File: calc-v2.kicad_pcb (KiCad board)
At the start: 2 copper layers, 32 parts, among them U1 W25Q128JVS, U2 NCP1117-3.3_SOT223, U3 BQ24074RGT, U4 TPS61165DBV, U5 RP2350B, U6 APS6404L-3SQRx-ZR

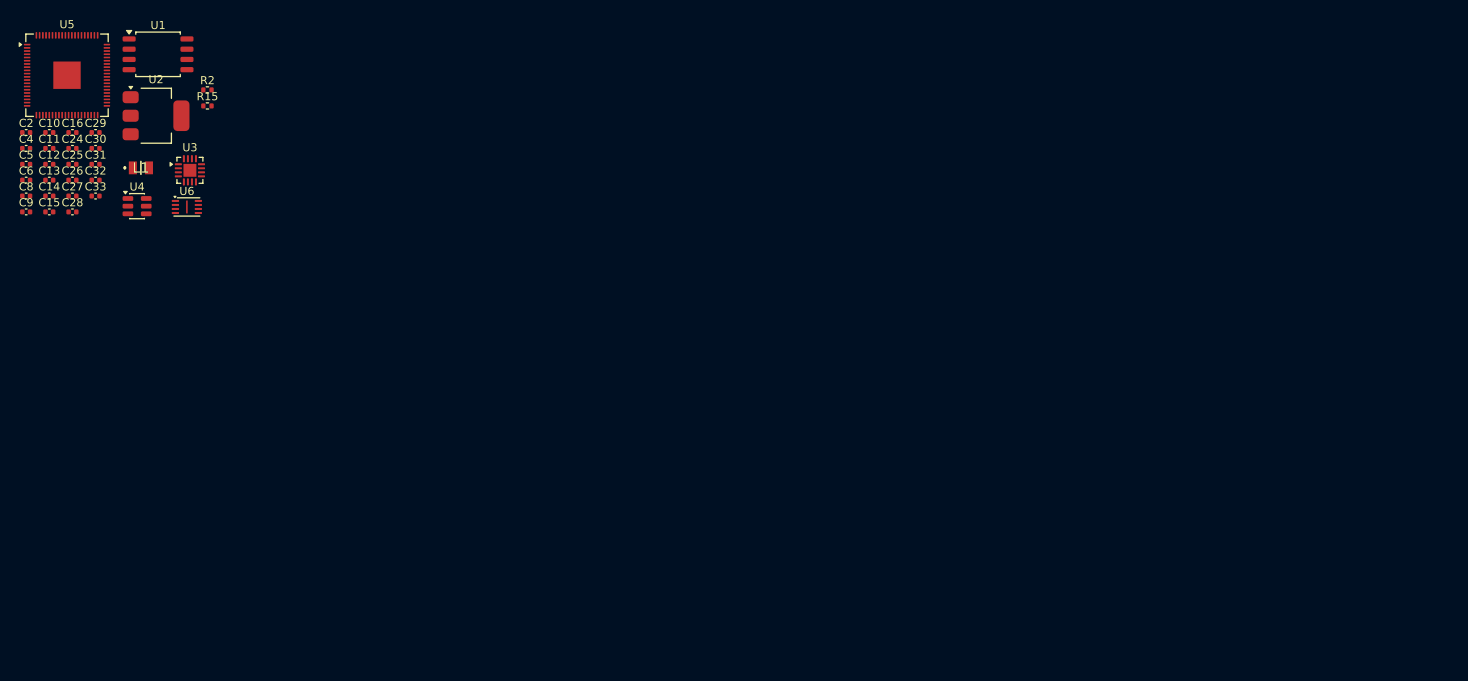
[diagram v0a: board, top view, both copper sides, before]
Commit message: more changes
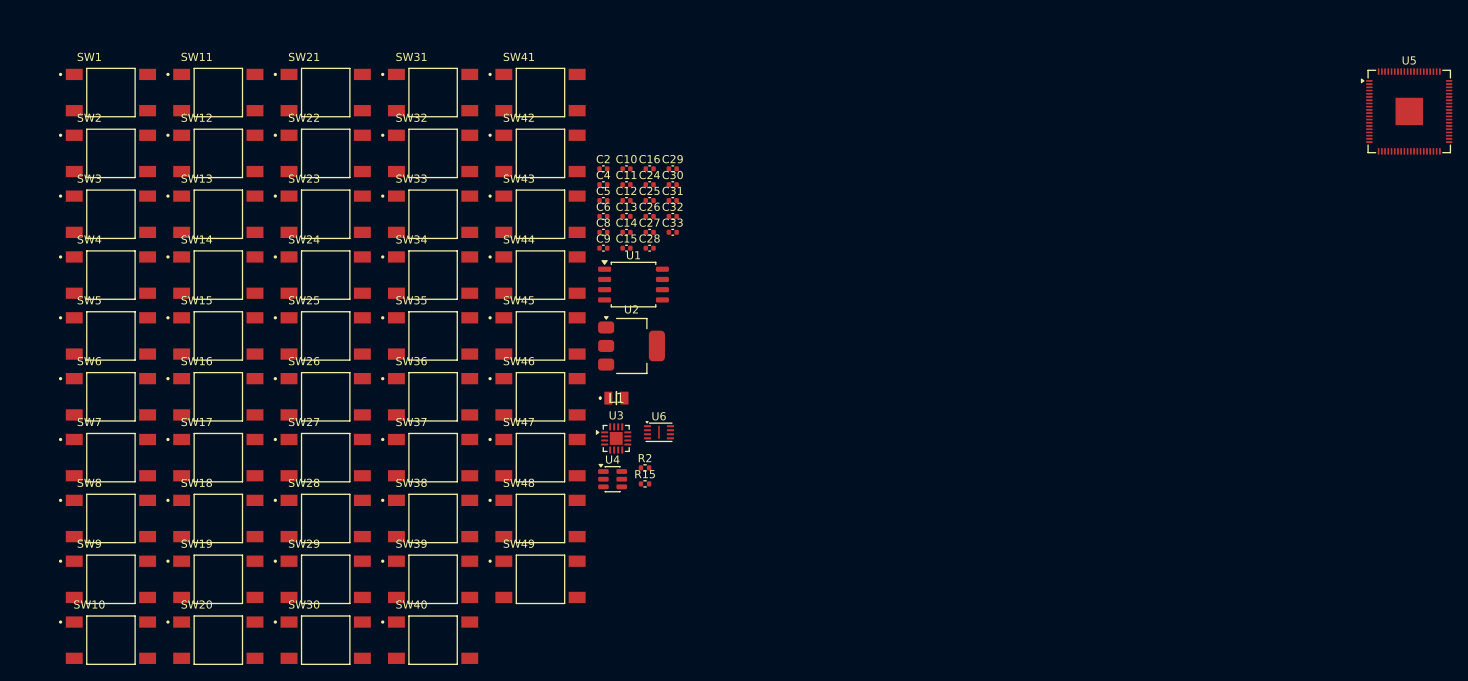
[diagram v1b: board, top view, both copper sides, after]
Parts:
- added SW1: TS04-66-43-BK-100-SMT, AAAAA:SW_TS04-66-43-BK-100-SMT, F.Cu at (23.9, 20.3)
- added SW10: TS04-66-43-BK-100-SMT, AAAAA:SW_TS04-66-43-BK-100-SMT, F.Cu at (23.9, 88.2)
- added SW11: TS04-66-43-BK-100-SMT, AAAAA:SW_TS04-66-43-BK-100-SMT, F.Cu at (37.3, 20.3)
- added SW12: TS04-66-43-BK-100-SMT, AAAAA:SW_TS04-66-43-BK-100-SMT, F.Cu at (37.3, 27.8)
- added SW13: TS04-66-43-BK-100-SMT, AAAAA:SW_TS04-66-43-BK-100-SMT, F.Cu at (37.3, 35.4)
- added SW14: TS04-66-43-BK-100-SMT, AAAAA:SW_TS04-66-43-BK-100-SMT, F.Cu at (37.3, 42.9)
- added SW15: TS04-66-43-BK-100-SMT, AAAAA:SW_TS04-66-43-BK-100-SMT, F.Cu at (37.3, 50.5)
- added SW16: TS04-66-43-BK-100-SMT, AAAAA:SW_TS04-66-43-BK-100-SMT, F.Cu at (37.3, 58.0)
- added SW17: TS04-66-43-BK-100-SMT, AAAAA:SW_TS04-66-43-BK-100-SMT, F.Cu at (37.3, 65.6)
- added SW18: TS04-66-43-BK-100-SMT, AAAAA:SW_TS04-66-43-BK-100-SMT, F.Cu at (37.3, 73.1)
- added SW19: TS04-66-43-BK-100-SMT, AAAAA:SW_TS04-66-43-BK-100-SMT, F.Cu at (37.3, 80.7)
- added SW2: TS04-66-43-BK-100-SMT, AAAAA:SW_TS04-66-43-BK-100-SMT, F.Cu at (23.9, 27.8)
- added SW20: TS04-66-43-BK-100-SMT, AAAAA:SW_TS04-66-43-BK-100-SMT, F.Cu at (37.3, 88.2)
- added SW21: TS04-66-43-BK-100-SMT, AAAAA:SW_TS04-66-43-BK-100-SMT, F.Cu at (50.6, 20.3)
- added SW22: TS04-66-43-BK-100-SMT, AAAAA:SW_TS04-66-43-BK-100-SMT, F.Cu at (50.6, 27.8)
- added SW23: TS04-66-43-BK-100-SMT, AAAAA:SW_TS04-66-43-BK-100-SMT, F.Cu at (50.6, 35.4)
- added SW24: TS04-66-43-BK-100-SMT, AAAAA:SW_TS04-66-43-BK-100-SMT, F.Cu at (50.6, 42.9)
- added SW25: TS04-66-43-BK-100-SMT, AAAAA:SW_TS04-66-43-BK-100-SMT, F.Cu at (50.6, 50.5)
- added SW26: TS04-66-43-BK-100-SMT, AAAAA:SW_TS04-66-43-BK-100-SMT, F.Cu at (50.6, 58.0)
- added SW27: TS04-66-43-BK-100-SMT, AAAAA:SW_TS04-66-43-BK-100-SMT, F.Cu at (50.6, 65.6)
- added SW28: TS04-66-43-BK-100-SMT, AAAAA:SW_TS04-66-43-BK-100-SMT, F.Cu at (50.6, 73.1)
- added SW29: TS04-66-43-BK-100-SMT, AAAAA:SW_TS04-66-43-BK-100-SMT, F.Cu at (50.6, 80.7)
- added SW3: TS04-66-43-BK-100-SMT, AAAAA:SW_TS04-66-43-BK-100-SMT, F.Cu at (23.9, 35.4)
- added SW30: TS04-66-43-BK-100-SMT, AAAAA:SW_TS04-66-43-BK-100-SMT, F.Cu at (50.6, 88.2)
- added SW31: TS04-66-43-BK-100-SMT, AAAAA:SW_TS04-66-43-BK-100-SMT, F.Cu at (63.9, 20.3)
- added SW32: TS04-66-43-BK-100-SMT, AAAAA:SW_TS04-66-43-BK-100-SMT, F.Cu at (63.9, 27.8)
- added SW33: TS04-66-43-BK-100-SMT, AAAAA:SW_TS04-66-43-BK-100-SMT, F.Cu at (63.9, 35.4)
- added SW34: TS04-66-43-BK-100-SMT, AAAAA:SW_TS04-66-43-BK-100-SMT, F.Cu at (63.9, 42.9)
- added SW35: TS04-66-43-BK-100-SMT, AAAAA:SW_TS04-66-43-BK-100-SMT, F.Cu at (63.9, 50.5)
- added SW36: TS04-66-43-BK-100-SMT, AAAAA:SW_TS04-66-43-BK-100-SMT, F.Cu at (63.9, 58.0)
- added SW37: TS04-66-43-BK-100-SMT, AAAAA:SW_TS04-66-43-BK-100-SMT, F.Cu at (63.9, 65.6)
- added SW38: TS04-66-43-BK-100-SMT, AAAAA:SW_TS04-66-43-BK-100-SMT, F.Cu at (63.9, 73.1)
- added SW39: TS04-66-43-BK-100-SMT, AAAAA:SW_TS04-66-43-BK-100-SMT, F.Cu at (63.9, 80.7)
- added SW4: TS04-66-43-BK-100-SMT, AAAAA:SW_TS04-66-43-BK-100-SMT, F.Cu at (23.9, 42.9)
- added SW40: TS04-66-43-BK-100-SMT, AAAAA:SW_TS04-66-43-BK-100-SMT, F.Cu at (63.9, 88.2)
- added SW41: TS04-66-43-BK-100-SMT, AAAAA:SW_TS04-66-43-BK-100-SMT, F.Cu at (77.2, 20.3)
- added SW42: TS04-66-43-BK-100-SMT, AAAAA:SW_TS04-66-43-BK-100-SMT, F.Cu at (77.2, 27.8)
- added SW43: TS04-66-43-BK-100-SMT, AAAAA:SW_TS04-66-43-BK-100-SMT, F.Cu at (77.2, 35.4)
- added SW44: TS04-66-43-BK-100-SMT, AAAAA:SW_TS04-66-43-BK-100-SMT, F.Cu at (77.2, 42.9)
- added SW45: TS04-66-43-BK-100-SMT, AAAAA:SW_TS04-66-43-BK-100-SMT, F.Cu at (77.2, 50.5)
- added SW46: TS04-66-43-BK-100-SMT, AAAAA:SW_TS04-66-43-BK-100-SMT, F.Cu at (77.2, 58.0)
- added SW47: TS04-66-43-BK-100-SMT, AAAAA:SW_TS04-66-43-BK-100-SMT, F.Cu at (77.2, 65.6)
- added SW48: TS04-66-43-BK-100-SMT, AAAAA:SW_TS04-66-43-BK-100-SMT, F.Cu at (77.2, 73.1)
- added SW49: SW_Push_45deg, AAAAA:SW_TS04-66-43-BK-100-SMT, F.Cu at (77.2, 80.7)
- added SW5: TS04-66-43-BK-100-SMT, AAAAA:SW_TS04-66-43-BK-100-SMT, F.Cu at (23.9, 50.5)
- added SW6: TS04-66-43-BK-100-SMT, AAAAA:SW_TS04-66-43-BK-100-SMT, F.Cu at (23.9, 58.0)
- added SW7: TS04-66-43-BK-100-SMT, AAAAA:SW_TS04-66-43-BK-100-SMT, F.Cu at (23.9, 65.6)
- added SW8: TS04-66-43-BK-100-SMT, AAAAA:SW_TS04-66-43-BK-100-SMT, F.Cu at (23.9, 73.1)
- added SW9: TS04-66-43-BK-100-SMT, AAAAA:SW_TS04-66-43-BK-100-SMT, F.Cu at (23.9, 80.7)
- moved U5 166.6 mm to (185.1, 22.6)
- moved C10 71.8 mm to (87.9, 29.7)
- moved C11 71.8 mm to (87.9, 31.7)
- moved C12 71.8 mm to (87.9, 33.7)
- moved C13 71.8 mm to (87.9, 35.6)
- moved C14 71.8 mm to (87.9, 37.6)
- moved C15 71.8 mm to (87.9, 39.6)
- moved C16 71.8 mm to (90.8, 29.7)
- moved C2 71.8 mm to (85.1, 29.7)
- moved C24 71.8 mm to (90.8, 31.7)
- moved C25 71.8 mm to (90.8, 33.7)
- moved C26 71.8 mm to (90.8, 35.6)
- moved C27 71.8 mm to (90.8, 37.6)
- moved C28 71.8 mm to (90.8, 39.6)
- moved C29 71.8 mm to (93.7, 29.7)
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
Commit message: components
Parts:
- added C34: 1u, Capacitor_SMD:C_0402_1005Metric, F.Cu at (202.6, 60.5)
- SW1, SW10, SW11, SW12, SW13, SW14, SW15, SW16, SW17, SW18, SW19, SW2, SW20, SW21, SW22, SW23, SW24, SW25, SW26, SW27, SW28, SW29, SW3, SW30, SW31, SW32, SW33, SW34, SW35, SW36, SW37, SW38, SW39, SW4, SW40, SW41, SW42, SW43, SW44, SW45, SW46, SW47, SW48, SW5, SW6, SW7, SW8, SW9: value TS04-66-43-BK-100-SMT -> SW_Push_45deg
- moved SW43 233.3 mm to (310.4, 30.0)
- moved SW44 219.5 mm to (296.4, 30.0)
- moved SW45 206.0 mm to (282.3, 30.0)
- moved SW46 193.0 mm to (268.2, 30.0)
- moved SW47 180.4 mm to (254.1, 30.0)
- moved SW48 168.4 mm to (240.0, 30.0)
- moved SW36 125.1 mm to (181.4, 101.0)
- moved SW16 125.1 mm to (154.8, 101.0)
- moved SW26 125.1 mm to (168.1, 101.0)
- moved SW1 125.1 mm to (141.4, 63.3)
- moved SW10 125.1 mm to (141.4, 131.2)
- moved SW2 125.1 mm to (141.4, 70.8)
- moved SW3 125.1 mm to (141.4, 78.4)
- moved SW31 125.1 mm to (181.4, 63.3)
- moved SW32 125.1 mm to (181.4, 70.8)
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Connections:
- SW1 pad 2: Net-(SW1-Pad2) -> SW_R1
- SW10 pad 1: Net-(SW10-Pad1) -> SW_C4
- SW10 pad 2: Net-(SW10-Pad2) -> SW_R2
- SW11 pad 1: Net-(SW11-Pad1) -> SW_C5
- SW11 pad 2: Net-(SW11-Pad2) -> SW_R2
- SW12 pad 2: unconnected-(SW12-Pad2) -> SW_R2
- SW13 pad 1: Net-(SW13-Pad1) -> SW_C1
- SW13 pad 2: Net-(SW13-Pad2) -> SW_R3
- SW14 pad 1: Net-(SW14-Pad1) -> SW_C2
- SW14 pad 2: Net-(SW14-Pad2) -> SW_R3
- SW15 pad 1: Net-(SW15-Pad1) -> SW_C3
- SW15 pad 2: Net-(SW15-Pad2) -> SW_R3
- SW16 pad 1: Net-(SW10-Pad3) -> SW_C4
- SW16 pad 2: Net-(SW16-Pad2) -> SW_R3
- SW17 pad 1: Net-(SW11-Pad3) -> SW_C5
- SW17 pad 2: Net-(SW17-Pad2) -> SW_R3
- SW18 pad 1: Net-(SW12-Pad3) -> Net-(SW12-Pad1)
- SW18 pad 2: unconnected-(SW18-Pad2) -> SW_R3
- SW19 pad 1: Net-(SW13-Pad3) -> SW_C1
- SW19 pad 2: Net-(SW19-Pad2) -> SW_R4
- SW2 pad 2: Net-(SW2-Pad2) -> SW_R1
- SW20 pad 1: Net-(SW14-Pad3) -> SW_C2
- SW20 pad 2: Net-(SW20-Pad2) -> SW_R4
- SW21 pad 1: Net-(SW15-Pad3) -> SW_C3
- SW21 pad 2: Net-(SW21-Pad2) -> SW_R4
- SW22 pad 1: Net-(SW16-Pad3) -> SW_C4
- SW22 pad 2: Net-(SW22-Pad2) -> SW_R4
- SW23 pad 1: Net-(SW17-Pad3) -> SW_C5
- SW23 pad 2: Net-(SW23-Pad2) -> SW_R4
- SW24 pad 1: Net-(SW18-Pad3) -> Net-(SW12-Pad1)
- SW24 pad 2: unconnected-(SW24-Pad2) -> SW_R4
- SW25 pad 1: Net-(SW19-Pad3) -> SW_C1
- SW25 pad 2: Net-(SW25-Pad2) -> SW_R5
- SW26 pad 1: Net-(SW20-Pad3) -> SW_C2
- SW26 pad 2: Net-(SW26-Pad2) -> SW_R5
- SW27 pad 1: Net-(SW21-Pad3) -> SW_C3
- SW27 pad 2: Net-(SW27-Pad2) -> SW_R5
- SW28 pad 1: Net-(SW22-Pad3) -> SW_C4
- SW28 pad 2: Net-(SW28-Pad2) -> SW_R5
- SW29 pad 1: Net-(SW23-Pad3) -> SW_C5
- SW29 pad 2: Net-(SW29-Pad2) -> SW_R5
- SW3 pad 2: Net-(SW3-Pad2) -> SW_R1
- SW30 pad 1: Net-(SW24-Pad3) -> Net-(SW12-Pad1)
- SW30 pad 2: unconnected-(SW30-Pad2) -> SW_R5
- SW31 pad 1: Net-(SW25-Pad3) -> SW_C1
- SW31 pad 2: Net-(SW31-Pad2) -> SW_R6
- SW32 pad 1: Net-(SW26-Pad3) -> SW_C2
- SW32 pad 2: Net-(SW32-Pad2) -> SW_R6
- SW33 pad 1: Net-(SW27-Pad3) -> SW_C3
- SW33 pad 2: Net-(SW33-Pad2) -> SW_R6
- SW34 pad 1: Net-(SW28-Pad3) -> SW_C4
- SW34 pad 2: Net-(SW34-Pad2) -> SW_R6
- SW35 pad 1: Net-(SW29-Pad3) -> SW_C5
- SW35 pad 2: Net-(SW35-Pad2) -> SW_R6
- SW36 pad 1: Net-(SW30-Pad3) -> Net-(SW12-Pad1)
- SW36 pad 2: unconnected-(SW36-Pad2) -> SW_R6
- SW37 pad 1: Net-(SW31-Pad3) -> SW_C1
- SW37 pad 2: Net-(SW37-Pad2) -> SW_R7
- SW38 pad 1: Net-(SW32-Pad3) -> SW_C2
- SW38 pad 2: Net-(SW38-Pad2) -> SW_R7
- SW39 pad 1: Net-(SW33-Pad3) -> SW_C3
- SW39 pad 2: Net-(SW39-Pad2) -> SW_R7
- SW4 pad 2: Net-(SW4-Pad2) -> SW_R1
- SW40 pad 1: Net-(SW34-Pad3) -> SW_C4
- SW40 pad 2: Net-(SW40-Pad2) -> SW_R7
- SW41 pad 1: Net-(SW35-Pad3) -> SW_C5
- SW41 pad 2: Net-(SW41-Pad2) -> SW_R7
- SW42 pad 1: Net-(SW36-Pad3) -> Net-(SW12-Pad1)
- SW42 pad 2: unconnected-(SW42-Pad2) -> SW_R7
- SW43 pad 1: Net-(SW37-Pad3) -> SW_C1
- SW43 pad 2: Net-(SW43-Pad2) -> SW_R8
- SW44 pad 1: Net-(SW38-Pad3) -> SW_C2
- SW44 pad 2: Net-(SW44-Pad2) -> SW_R8
- SW45 pad 1: Net-(SW39-Pad3) -> SW_C3
- SW45 pad 2: Net-(SW45-Pad2) -> SW_R8
- SW46 pad 1: Net-(SW40-Pad3) -> SW_C4
- SW46 pad 2: Net-(SW46-Pad2) -> SW_R8
- SW47 pad 1: Net-(SW41-Pad3) -> SW_C5
- SW47 pad 2: Net-(SW47-Pad2) -> SW_R8
- SW48 pad 1: Net-(SW42-Pad3) -> Net-(SW12-Pad1)
- SW48 pad 2: unconnected-(SW48-Pad2) -> SW_R8
- SW5 pad 2: Net-(SW5-Pad2) -> SW_R1
- SW6 pad 1: SW_C6 -> Net-(SW12-Pad1)
- SW6 pad 2: unconnected-(SW6-Pad2) -> SW_R1
- SW7 pad 1: Net-(SW1-Pad3) -> SW_C1
- SW7 pad 2: Net-(SW7-Pad2) -> SW_R2
- SW8 pad 1: Net-(SW2-Pad3) -> SW_C2
- SW8 pad 2: Net-(SW8-Pad2) -> SW_R2
- SW9 pad 1: Net-(SW3-Pad3) -> SW_C3
- SW9 pad 2: Net-(SW10-Pad4) -> SW_R2
- U3 pad 13: unconnected-(U3-IN-Pad13) -> VBUS
- U6 pad 9: unconnected-(U6-EPAD-Pad9) -> GND
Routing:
- net SW_R8: track 0.00 -> 24.9 mm
